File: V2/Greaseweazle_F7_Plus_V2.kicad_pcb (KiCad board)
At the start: 2 copper layers, 80 x 50 mm, 71 parts, among them J1 Wurth 694106301002, J10 PIN1X2, J11 PIN1X2, J12 IDC Box Header, J2 USB_B, J3 Molex 105017-1001, J4 TE EI 171826-4, J5 PIN1X3, J6 PIN1X2, J7 PIN1X5, J8 PIN1X4, J9 PIN1X4, Q1 SI2369DS-T1-GE3, U1 TPS562201DDC, U11 NarrowPowerAdapter, U12 NarrowPowerAdapter, U13 NarrowPowerAdapter, U15 NarrowPowerAdapter, U2 TLV75533PDBV, U3 TPUSBLC6-2SC6, U4 STM32F730R8T6, U5 74LVC07APW,118, U6 74LVC07APW,118, U7 NarrowPowerAdapter, U8 NarrowPowerAdapter, U9 NarrowPowerAdapter, Y1 8.000MHz

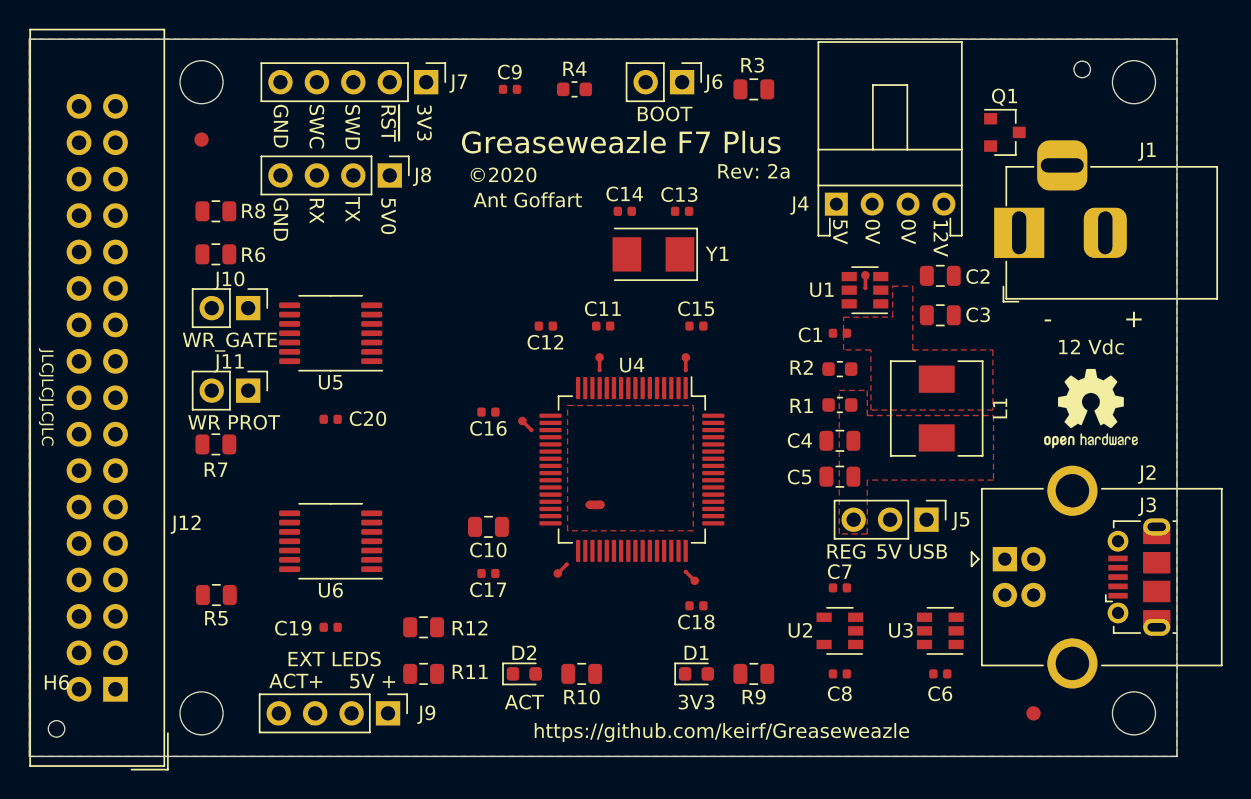
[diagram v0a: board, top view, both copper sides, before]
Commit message: routed latest version
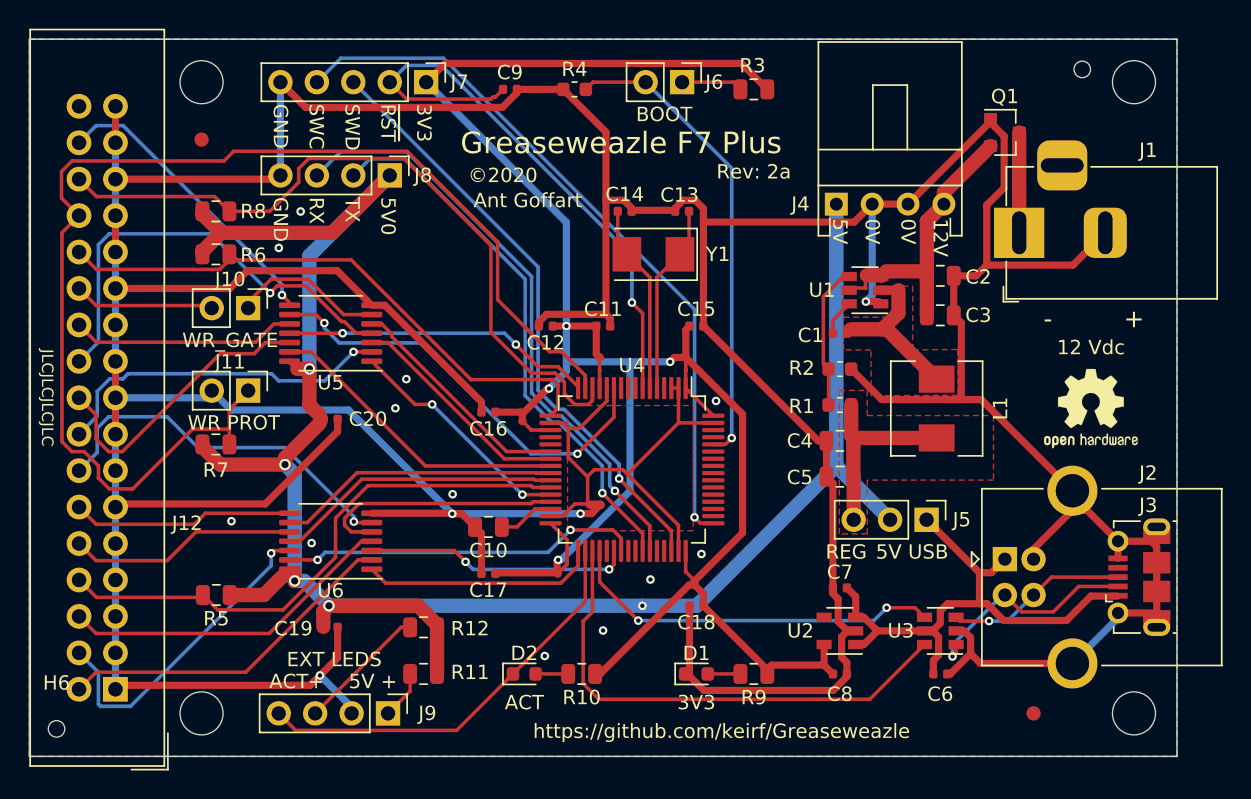
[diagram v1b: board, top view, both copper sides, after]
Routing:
- net GND: track 0.00 -> 407.7 mm, vias 0 -> 16
- net +5V: track 0.00 -> 143.1 mm, vias 0 -> 5
- net +3V3: track 0.00 -> 136.5 mm, vias 0 -> 4
- net /~WR_PROT~: track 0.00 -> 86.2 mm
- net /~RD_DAT~: track 0.00 -> 50.9 mm
- net /SWCLK: track 0.00 -> 50.2 mm, vias 0 -> 1
- net /SWDIO: track 0.00 -> 42.1 mm, vias 0 -> 1
- net /RX: track 0.00 -> 42.1 mm, vias 0 -> 1
- net /~RST~: track 0.00 -> 41.1 mm, vias 0 -> 1
- net /~TRK_00~: track 0.00 -> 40.5 mm
- net /~INDEX~: track 0.00 -> 39.1 mm
- net /TX: track 0.00 -> 38.6 mm, vias 0 -> 1
- net /USB_VBUS: track 0.00 -> 38.3 mm
- net /USB_D-: track 0.00 -> 35.3 mm
- net /GND_for_U4: track 0.00 -> 34.9 mm
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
